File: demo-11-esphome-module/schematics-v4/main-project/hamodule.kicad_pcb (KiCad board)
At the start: 2 copper layers, 54 parts, among them J1 1017505, J2 1017505, J4 1017505, K1 G5Q-1, K2 G5Q-1, K3 G5Q-1, K4 G5Q-1, Q1 2N2219, Q2 2N2219, Q3 2N2219, Q4 2N2219, U1 ESP32-DEVKITC-32D, U2 HCPL3700, U3 HCPL3700, U4 HCPL3700, U5 HCPL3700

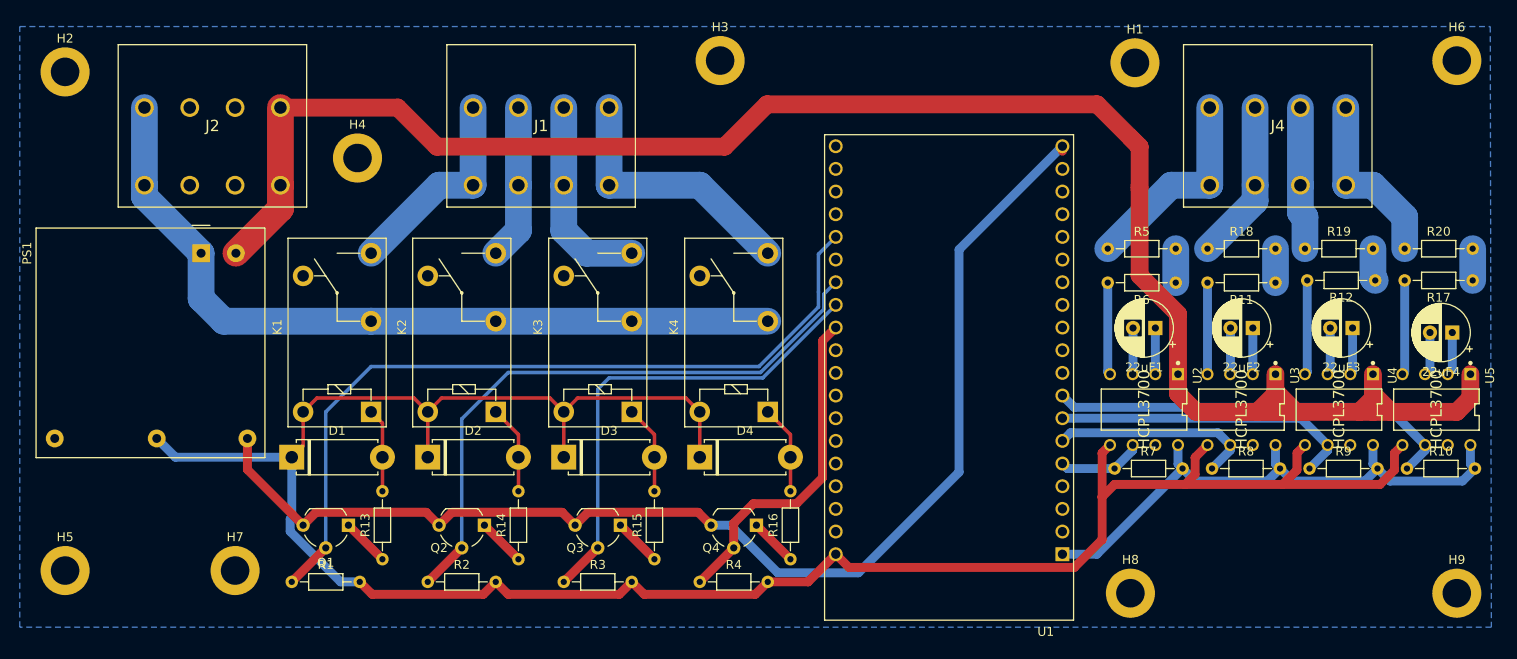
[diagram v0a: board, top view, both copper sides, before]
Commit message: some changes to schema
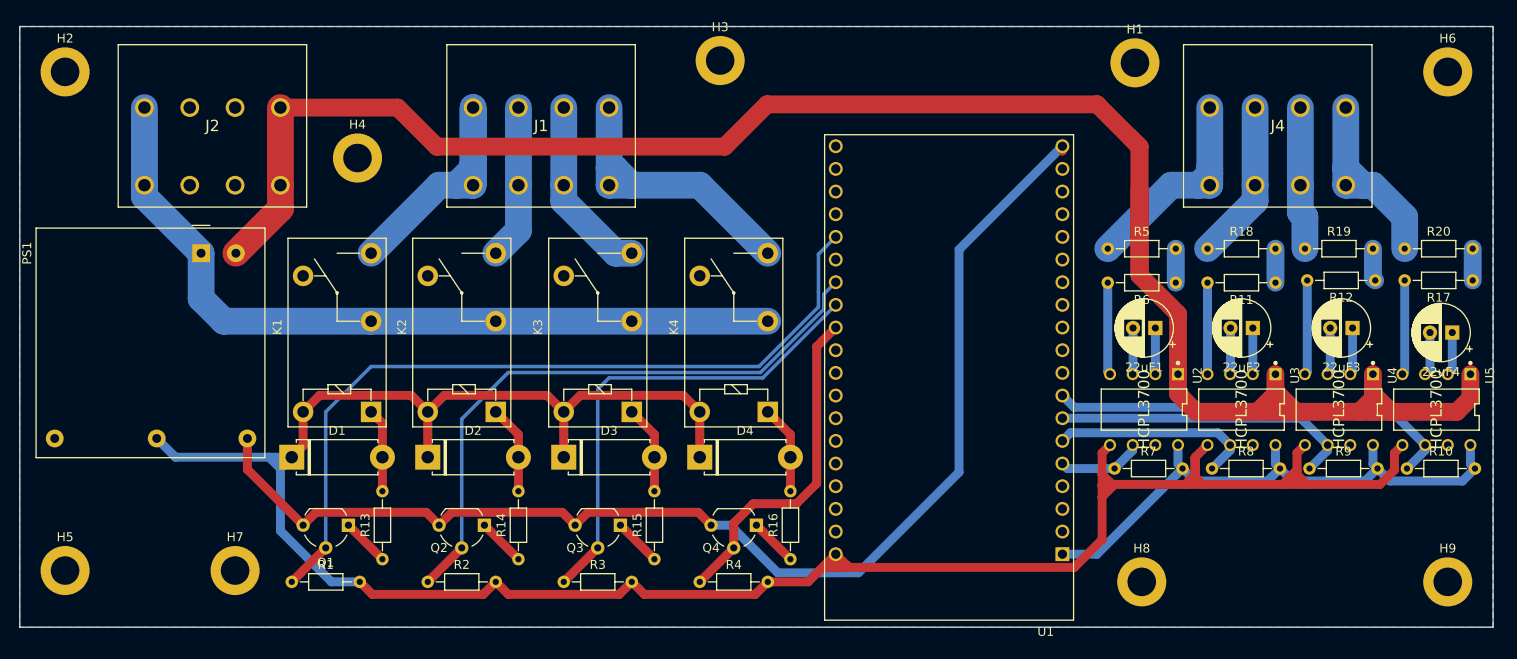
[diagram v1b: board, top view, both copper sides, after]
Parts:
- moved H8 1.80 mm to (147.3, 78.7)
- moved H9 1.63 mm to (181.6, 78.7)
- moved H6 1.63 mm to (181.6, 21.6)
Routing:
- net 5VGND: track 252.6 -> 274.1 mm
- net REO1: track 23.3 -> 35.3 mm
- net 220VAC(N): track 205.8 -> 215.7 mm
- net REO4: track 29.6 -> 33.0 mm
- net Sens4: track 20.3 -> 23.0 mm
- net Sens1: track 23.1 -> 25.5 mm
- net REO3: track 22.5 -> 20.5 mm
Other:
- board outline added: 165.1 x 67.3 mm
